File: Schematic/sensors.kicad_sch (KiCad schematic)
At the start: 17 parts, among them IC4 ICM-42688-P, IC5 MPU-6500, U5 SPL06-001, U7 QMC5883L

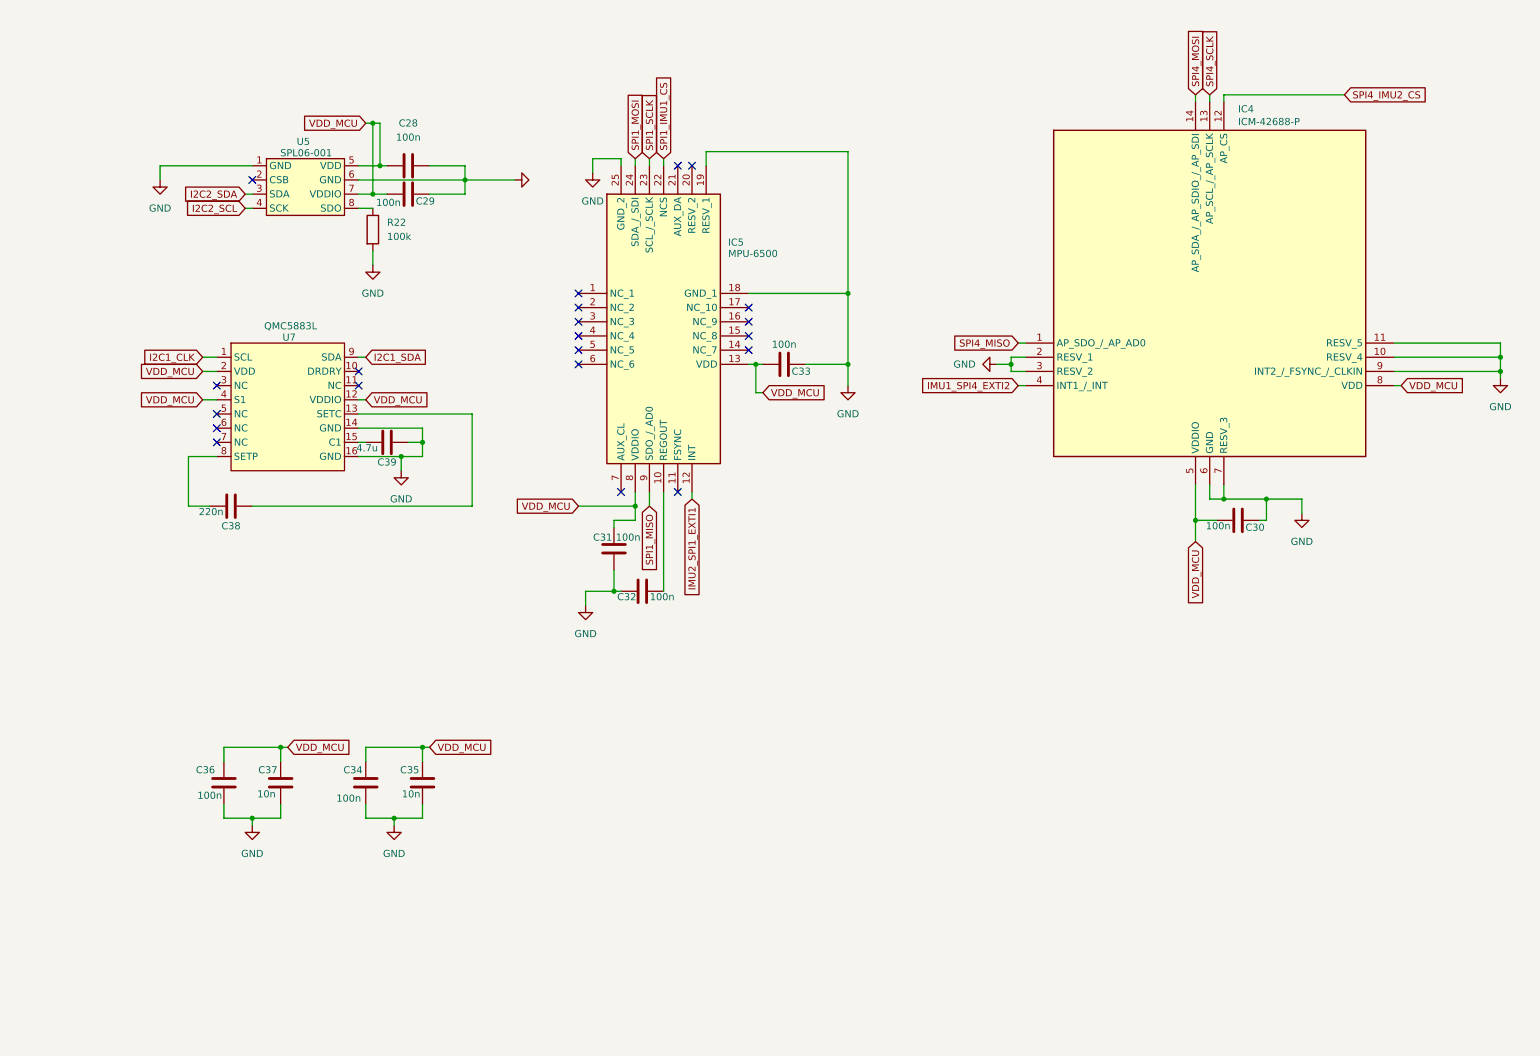
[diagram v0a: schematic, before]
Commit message: Refactor code structure for improved readability and maintainability
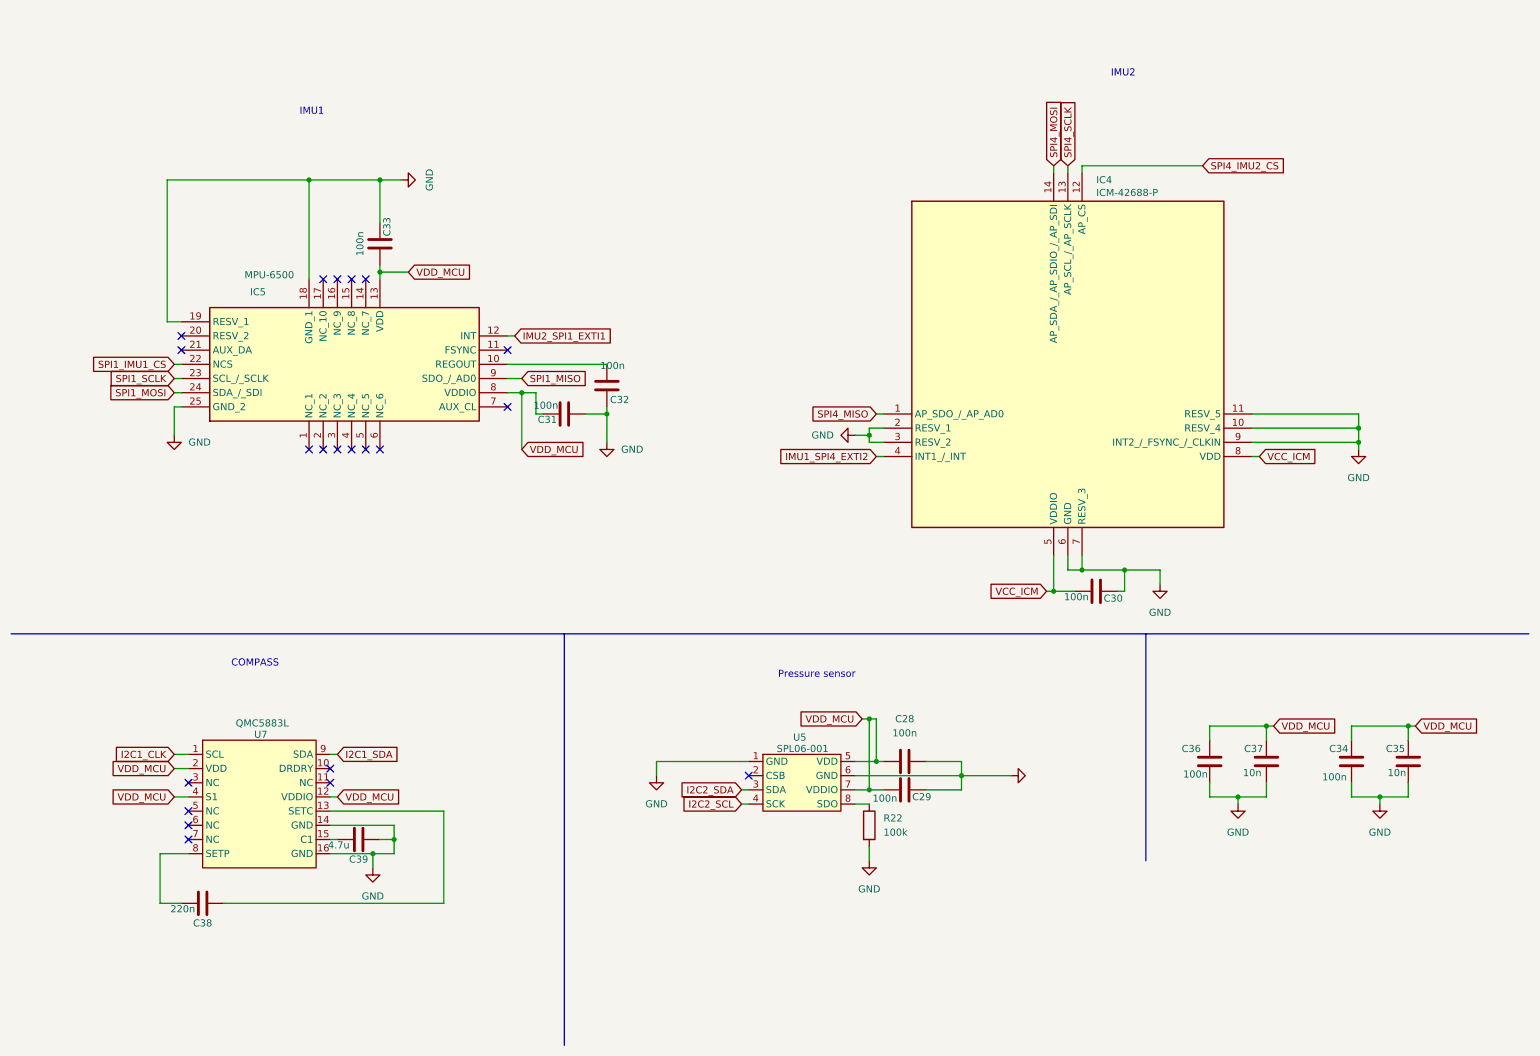
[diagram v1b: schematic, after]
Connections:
- net VDD_MCU: no longer C30.1, IC4.5 (VDDIO), IC4.8 (VDD)
- new net VCC_ICM: C30.1, IC4.5 (VDDIO), IC4.8 (VDD)
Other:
- note added: "COMPASS"
- note added: "IMU1"
- note added: "IMU2"
- note added: "Pressure sensor"
- moved on the sheet: C28, C29, C30, C31, C32, C33, C34, C35, C36, C37, C38, C39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
